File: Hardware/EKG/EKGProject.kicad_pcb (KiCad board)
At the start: 2 copper layers, 93.5 x 80.8 mm, 66 parts, among them J1 Screw_Terminal_01x01, J10 Conn_01x04, J2 Screw_Terminal_01x01, J3 Screw_Terminal_01x01, J4 Conn_01x01, J5 Screw_Terminal_01x01, J6 Screw_Terminal_01x01, J7 Conn_01x01, J8 Conn_01x12, J9 Conn_01x16, U1 MAX1726EUK18+, U2 MAX30003, U3 MAX30003, U4 MAX30003

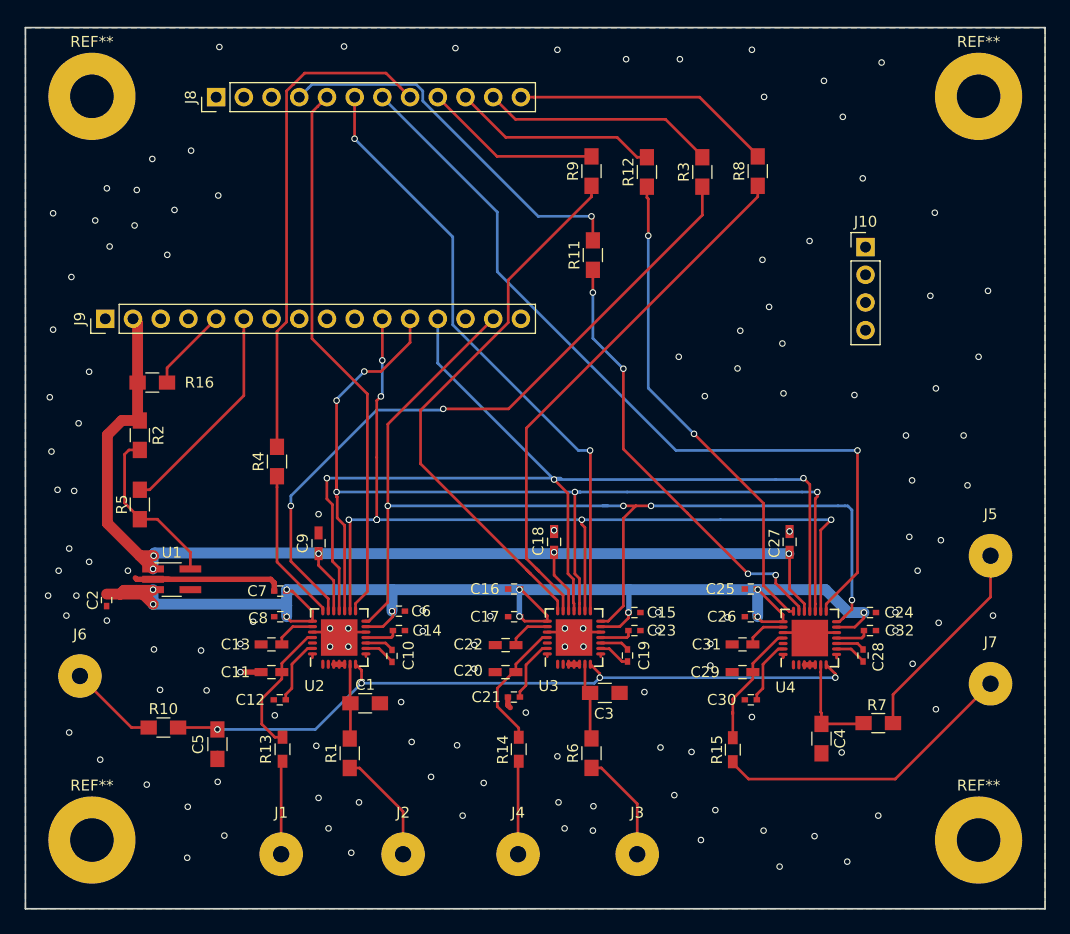
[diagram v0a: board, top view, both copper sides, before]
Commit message: DFM quick check
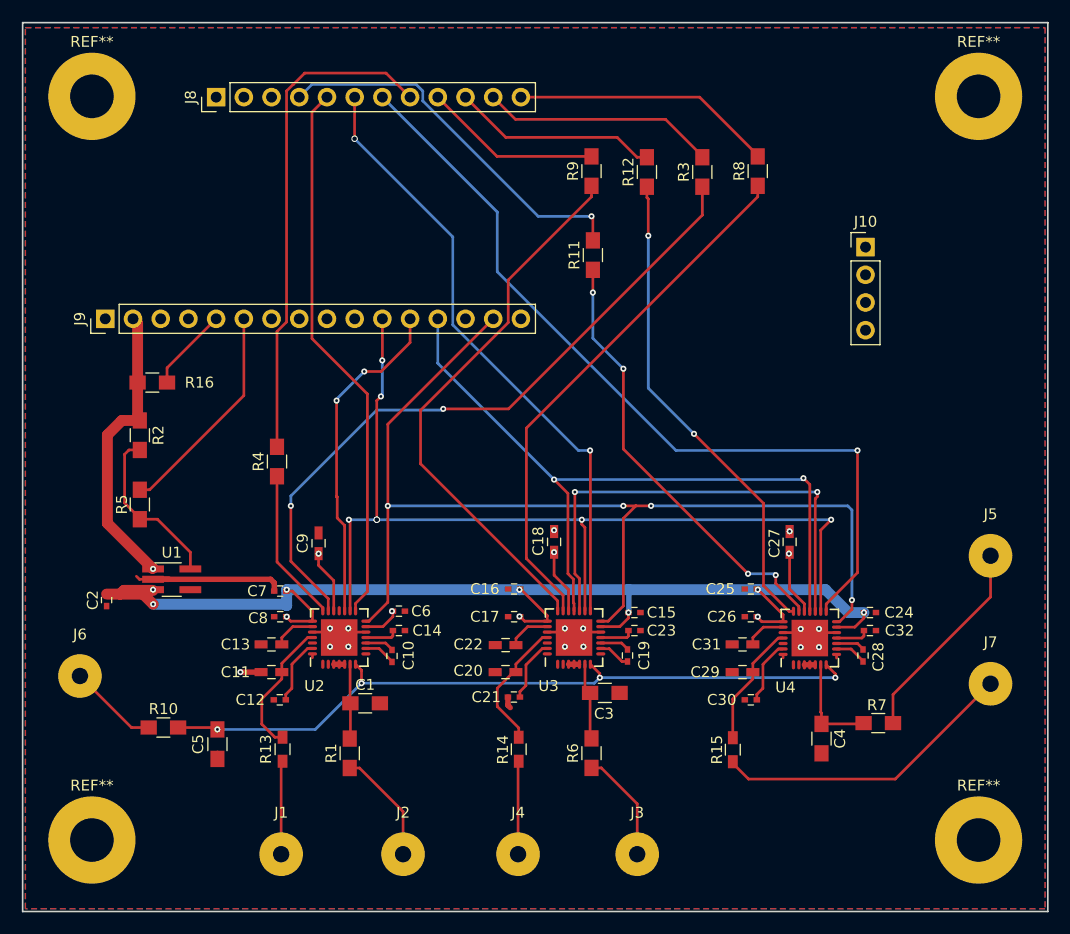
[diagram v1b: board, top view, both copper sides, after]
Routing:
- net +3V3: track 106.2 -> 45.2 mm, vias 5 -> 4
- net /MISO: track 101.6 -> 67.3 mm, vias 3 -> 2
- net /MOSI: track 98.1 -> 75.1 mm, vias 5 -> 4
- net +1V8: track 116.7 -> 107.5 mm
- net Earth: track 33.4 -> 32.3 mm, vias 133 -> 15
- net /FCLK: track 99.5 -> 98.7 mm
- net /INTB_2_R: track 51.2 -> 50.7 mm
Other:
- board size 93.5 x 80.8 mm -> 94 x 81.5 mm
